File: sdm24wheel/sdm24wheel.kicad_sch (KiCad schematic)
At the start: 47 parts, among them J1 ATM15-08PA, J2 SWD, J3 USB_B_Micro, SW1 BOOT, U1 STM32F072CBT6, U2 MLX90614, U3 MIC37100-3.3WS, U4 24LC01BT-E/LT, U5 SN65HVD230, U6 USBLC6-2SC6, Y1 8MHz

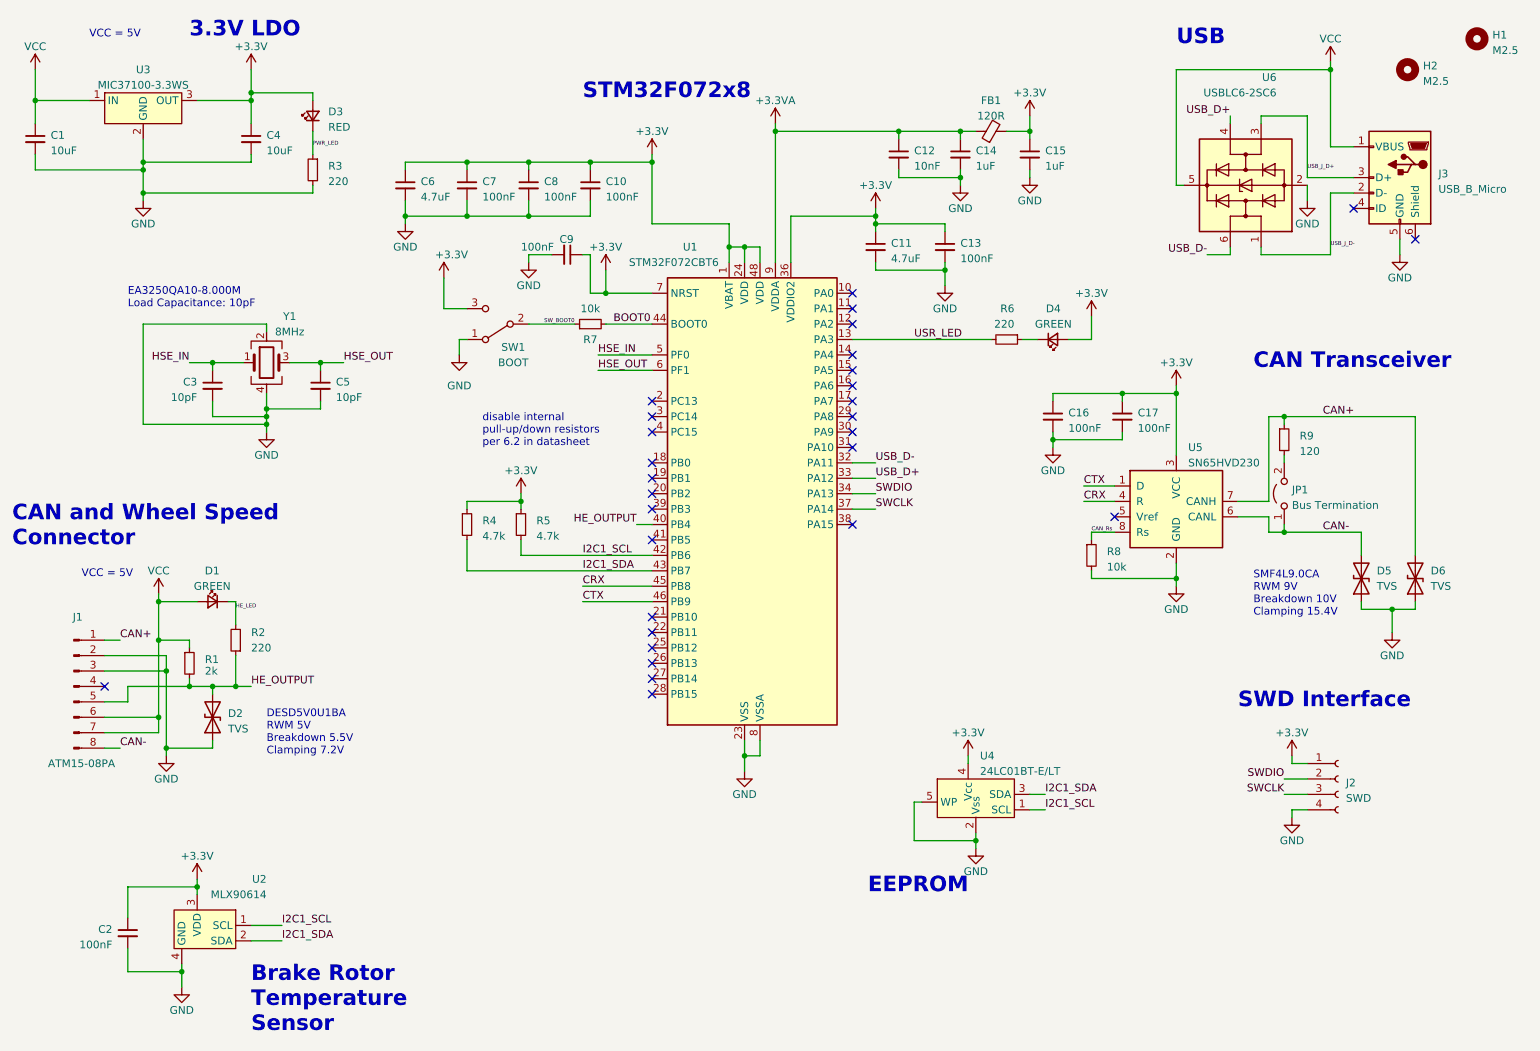
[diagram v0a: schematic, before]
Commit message: updating repo
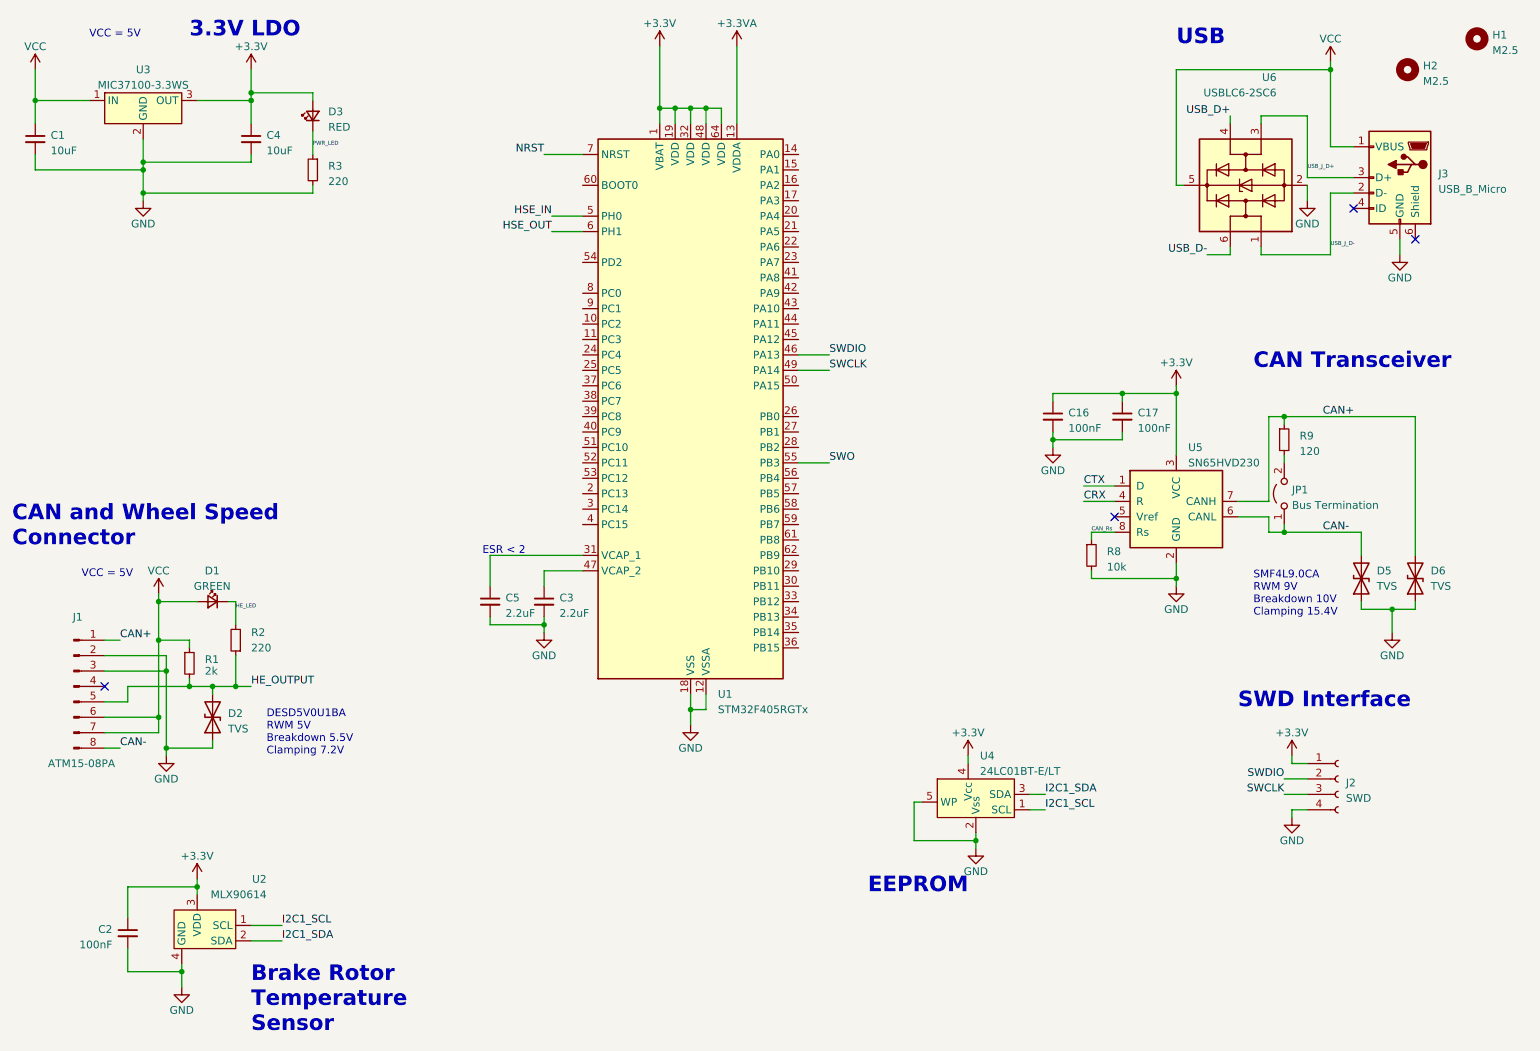
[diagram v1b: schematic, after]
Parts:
- removed C10, C13, C7, C8, C9: 100nF, Capacitor_SMD:C_0402_1005Metric, symbol Device:C_Small
- removed C11, C6: 4.7uF, Capacitor_SMD:C_0805_2012Metric, symbol Device:C_Small
- removed C12: 10nF, Capacitor_SMD:C_0402_1005Metric, symbol Device:C_Small
- removed C14, C15: 1uF, Capacitor_SMD:C_0805_2012Metric, symbol Device:C_Small
- removed D4: GREEN, Library:Dialight_561-XX0X-XXX, symbol Device:LED_Small
- removed FB1: 120R, Inductor_SMD:L_0603_1608Metric, symbol Device:FerriteBead_Small
- removed R4, R5: 4.7k, Resistor_SMD:R_0805_2012Metric, symbol Device:R_Small
- removed R6: 220, Resistor_SMD:R_0805_2012Metric, symbol Device:R_Small
- removed R7: 10k, Resistor_SMD:R_0805_2012Metric, symbol Device:R_Small
- removed SW1: BOOT, Library:Gravitech_MINI-SPDT-SW, symbol Switch:SW_SPDT
- removed U1: STM32F072CBT6, Package_QFP:LQFP-48_7x7mm_P0.5mm, symbol MCU_ST_STM32F0:STM32F072C8Tx
- removed Y1: 8MHz, Crystal:Crystal_SMD_Abracon_ABM3C-4Pin_5.0x3.2mm, symbol Device:Crystal_GND24
- added U1: STM32F405RGTx, Package_QFP:LQFP-64_10x10mm_P0.5mm, symbol MCU_ST_STM32F4:STM32F405RGTx
- C3, C5: value 10pF -> 2.2uF; footprint Capacitor_SMD:C_0603_1608Metric -> (none)
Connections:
- net +3.3V: now also U1.1 (VBAT), U1.19 (VDD), U1.32 (VDD), U1.48 (VDD), U1.64 (VDD)
- net +3.3VA: now also U1.13 (VDDA)
- net GND: now also U1.12 (VSSA), U1.18 (VSS), U1.63 (VSS)
- net HSE_IN: now also U1.5 (PH0); no longer C3.1
- net HSE_OUT: now also U1.6 (PH1); no longer C5.1
- net SWCLK: now also U1.49 (PA14)
- net SWDIO: now also U1.46 (PA13)
- new net: C5.1, U1.31 (VCAP_1)
- new net: C3.1, U1.47 (VCAP_2)
- new net NRST: U1.7 (NRST)
- new net SWO: U1.55 (PB3)
- no-connect marks 29 -> 4
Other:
- note added: "ESR < 2"
- note removed: "EA3250QA10-8.000M Load Capacitance: 10pF"
- note removed: "STM32F072x8"
- note removed: "disable internal pull-up/down resistors per 6.2 in datasheet"
